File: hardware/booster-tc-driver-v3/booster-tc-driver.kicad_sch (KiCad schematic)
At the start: 98 parts, among them IC1 CAT4109V-GT2, IC2 LDL1117S50R, J1 62201021121, J11 3-647166-5, J2 EHT-105-01-S-D, J3 22-23-2021, J4 3-647166-2, J5 3-647166-2, J6 3-647166-2, J7 3-647166-2, Q1 T2N7002AK, Q2 BUK9M5R2-30EX, SW1 SW_SPDT, U1 IF-D95T << must be T, U2 IF-E96E, U3 IF-D95T << must be T, U4 CSTNE8M00G550000R0, U5 STM32G474CBTx, U6 MCP9700Ax-ETT, U7 AP1501A-12K5G-13, U8 LT1963AxST-3.3

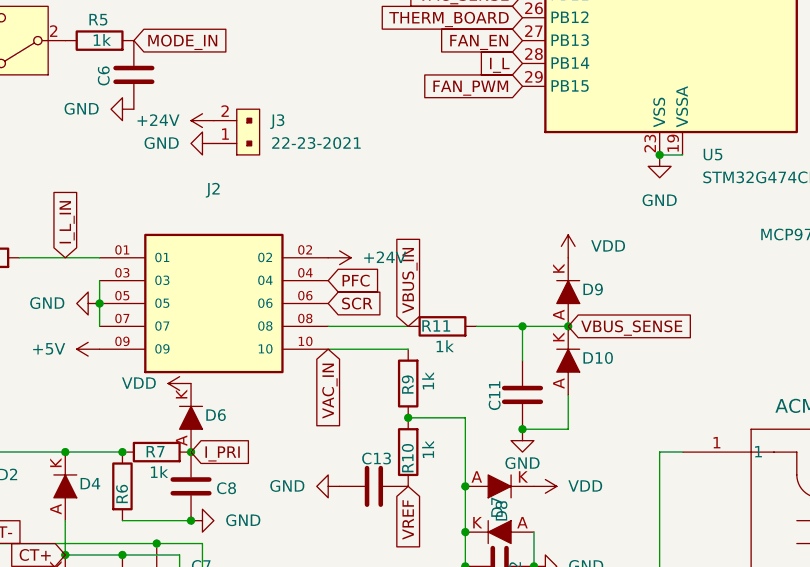
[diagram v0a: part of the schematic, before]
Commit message: pfc v3
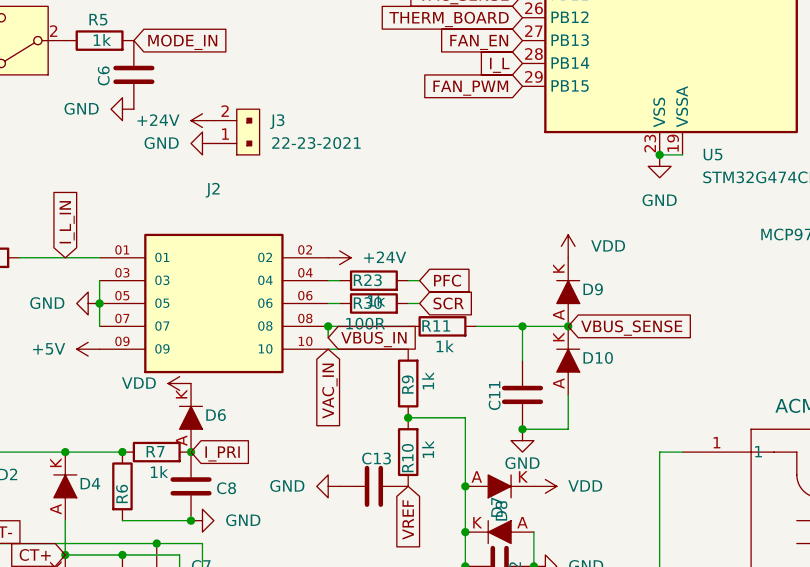
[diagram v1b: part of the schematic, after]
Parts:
- added R23: 1k, Resistor_SMD:R_0603_1608Metric_Pad0.98x0.95mm_HandSolder, symbol Device:R
- added R30: 100R, Resistor_SMD:R_0603_1608Metric_Pad0.98x0.95mm_HandSolder, symbol Device:R
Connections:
- net PFC: now also R23.2; no longer J2.04
- net SCR: now also R30.2; no longer J2.06
- new net: J2.06, R30.1
- new net: J2.04, R23.1
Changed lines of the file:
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@@
 	)
 	(junction
+		(at 62.23 160.02)
+		(diameter 0)
+		(color 0 0 0 0)
+	)
+	(junction
 		(at 36.83 53.34)
 		(diameter 0)
@@
 	(wire
 		(pts
+			(xy 71.12 157.48) (xy 72.39 157.48)
+		)
+		(stroke
+			(width 0)
+			(type default)
+		)
+	)
+	(wire
+		(pts
 			(xy 50.8 39.37) (xy 50.8 44.45)
 		)
@@
 	(wire
 		(pts
+			(xy 71.12 154.94) (xy 72.39 154.94)
+		)
+		(stroke
+			(width 0)
+			(type default)
+		)
+	)
+	(wire
+		(pts
 			(xy 99.06 140.97) (xy 101.6 140.97)
 		)
@@
 	(wire
 		(pts
+			(xy 62.23 157.48) (xy 63.5 157.48)
+		)
+		(stroke
+			(width 0)
+			(type default)
+		)
+	)
+	(wire
+		(pts
 			(xy 142.24 83.82) (xy 147.32 83.82)
 		)
@@
 	(wire
 		(pts
+			(xy 62.23 160.02) (xy 62.23 161.29)
+		)
+		(stroke
+			(width 0)
+			(type default)
+		)
+	)
+	(wire
+		(pts
 			(xy 39.37 181.61) (xy 46.99 181.61)
 		)
@@
 	(wire
 		(pts
+			(xy 62.23 154.94) (xy 63.5 154.94)
+		)
+		(stroke
+			(width 0)
+			(type default)
+		)
+	)
+	(wire
+		(pts
 			(xy 45.72 194.31) (xy 45.72 185.42)
 		)
@@
 		)
 	)
+	(global_label "PFC"
+		(shape input)
+		(at 72.39 154.94 0)
+		(fields_autoplaced yes)
+		(effects
+			(font
+				(size 1.27 1.27)
+			)
+			(justify left)
+		)
+		(property "Intersheetrefs" "${INTERSHEET_REFS}"
+			(at 79.0038 154.94 0)
+			(effects
+				(font
+					(size 1.27 1.27)
+				)
+				(justify left)
+				(hide yes)
+			)
+		)
+	)
 	(global_label "USART_TX"
 		(shape input)
@@
 		)
 	)
-	(global_label "VBUS_IN"
+	(global_label "SCR"
 		(shape input)
-		(at 71.12 160.02 90)
+		(at 72.39 157.48 0)
 		(fields_autoplaced yes)
 		(effects
@@
 		)
 		(property "Intersheetrefs" "${INTERSHEET_REFS}"
-			(at 71.12 149.2333 90)
+			(at 79.1247 157.48 0)
 			(effects
 				(font
@@
 		)
 	)
-	(global_label "SCR"
-		(shape input)
-		(at 62.23 157.48 0)
-		(fields_autoplaced yes)
-		(effects
-			(font
-				(size 1.27 1.27)
-			)
-			(justify left)
-		)
-		(property "Intersheetrefs" "${INTERSHEET_REFS}"
-			(at 68.9647 157.48 0)
-			(effects
-				(font
-					(size 1.27 1.27)
-				)
-				(justify left)
-				(hide yes)
-			)
-		)
-	)
-	(global_label "PFC"
-		(shape input)
-		(at 62.23 154.94 0)
-		(fields_autoplaced yes)
-		(effects
-			(font
-				(size 1.27 1.27)
-			)
-			(justify left)
-		)
-		(property "Intersheetrefs" "${INTERSHEET_REFS}"
-			(at 68.8438 154.94 0)
-			(effects
-				(font
-					(size 1.27 1.27)
-				)
-				(justify left)
-				(hide yes)
-			)
-		)
-	)
 	(global_label "VBUS_SENSE"
 		(shape input)
@@
 		)
 	)
+	(global_label "VBUS_IN"
+		(shape input)
+		(at 62.23 161.29 0)
+		(fields_autoplaced yes)
+		(effects
+			(font
+				(size 1.27 1.27)
+			)
+			(justify left)
+		)
+		(property "Intersheetrefs" "${INTERSHEET_REFS}"
+			(at 73.0167 161.29 0)
+			(effects
+				(font
+					(size 1.27 1.27)
+				)
+				(justify left)
+				(hide yes)
+			)
+		)
+	)
 	(symbol
 		(lib_id "Device:C")
@@
 	)
 	(symbol
+		(lib_id "Device:R")
+		(at 67.31 157.48 90)
+		(unit 1)
+		(exclude_from_sim no)
+		(in_bom yes)
+		(on_board yes)
+		(dnp no)
+		(property "Reference" "R30"
+			(at 68.326 157.48 90)
+			(effects
+				(font
+					(size 1.27 1.27)
+				)
+				(justify left)
+			)
+		)
+		(property "Value" "100R"
+			(at 68.58 159.766 90)
+			(effects
+				(font
+					(size 1.27 1.27)
+				)
+				(justify left)
+			)
+		)
+		(property "Footprint" "Resistor_SMD:R_0603_1608Metric_Pad0.98x0.95mm_HandSolder"
+			(at 67.31 159.258 90)
+			(effects
+				(font
+					(size 1.27 1.27)
+				)
+				(hide yes)
+			)
+		)
+		(property "Datasheet" "~"
+			(at 67.31 157.48 0)
+			(effects
+				(font
+					(size 1.27 1.27)
+				)
+				(hide yes)
+			)
+		)
+		(property "Description" "Resistor"
+			(at 67.31 157.48 0)
+			(effects
+				(font
+					(size 1.27 1.27)
+				)
+				(hide yes)
+			)
+		)
+		(pin "1"
+		)
+		(pin "2"
+		)
+		(instances
+			(project "booster-tc-driver"
+				(path "/3c175d5e-f31a-4933-a865-8318878a5034"
+					(reference "R30")
+					(unit 1)
+				)
+			)
+		)
+	)
+	(symbol
 		(lib_id "Device:C")
 		(at 46.99 177.8 0)
@@
 					(unit 1)
 				)
+			)
+		)
+	)
+	(symbol
+		(lib_id "Device:R")
+		(at 67.31 154.94 90)
+		(unit 1)
+		(exclude_from_sim no)
+		(in_bom yes)
+		(on_board yes)
+		(dnp no)
+		(property "Reference" "R23"
+			(at 68.326 154.94 90)
+			(effects
+				(font
+					(size 1.27 1.27)
+				)
+				(justify left)
+			)
+		)
+		(property "Value" "1k"
+			(at 68.58 157.226 90)
+			(effects
+				(font
+					(size 1.27 1.27)
+				)
+				(justify left)
+			)
+		)
+		(property "Footprint" "Resistor_SMD:R_0603_1608Metric_Pad0.98x0.95mm_HandSolder"
+			(at 67.31 156.718 90)
+			(effects
+				(font
+					(size 1.27 1.27)
+				)
+				(hide yes)
+			)
+		)
+		(property "Datasheet" "~"
+			(at 67.31 154.94 0)
+			(effects
+				(font
+					(size 1.27 1.27)
+				)
+				(hide yes)
+			)
+		)
+		(property "Description" "Resistor"
+			(at 67.31 154.94 0)
+			(effects
+				(font
+					(size 1.27 1.27)
+				)
+				(hide yes)
+			)
+		)
+		(pin "1"
+		)
+		(pin "2"
+		)
+		(instances
+			(project "booster-tc-driver"
+				(path "/3c175d5e-f31a-4933-a865-8318878a5034"
+					(reference "R23")
+					(unit 1)
+				)

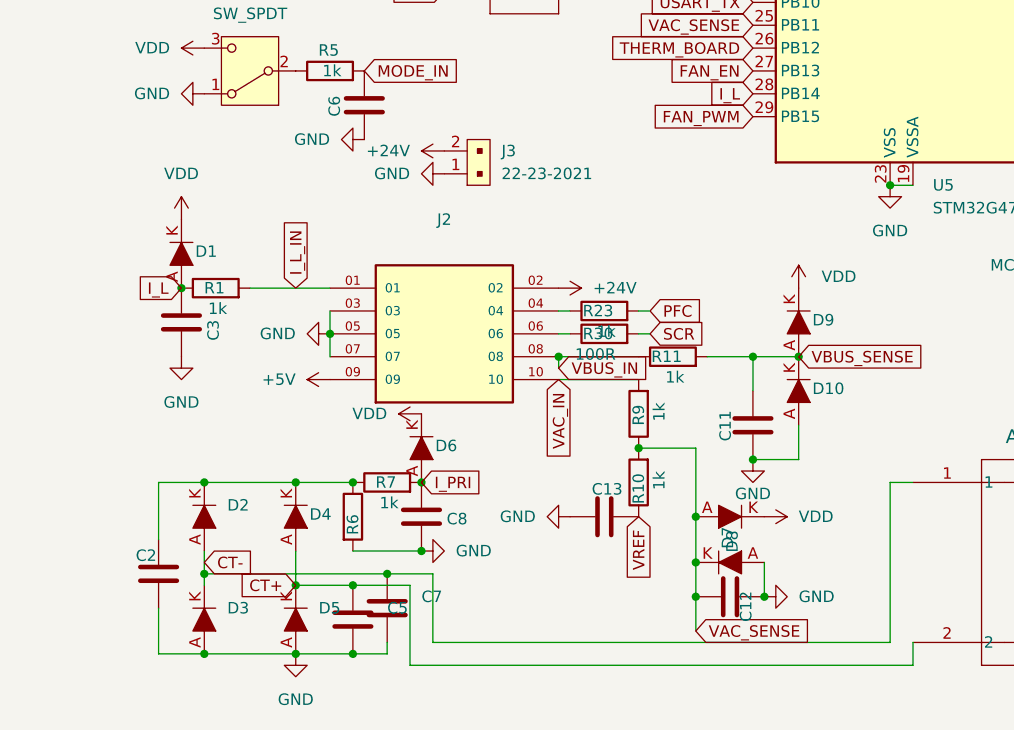
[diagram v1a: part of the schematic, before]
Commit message: pfc v3 finalized
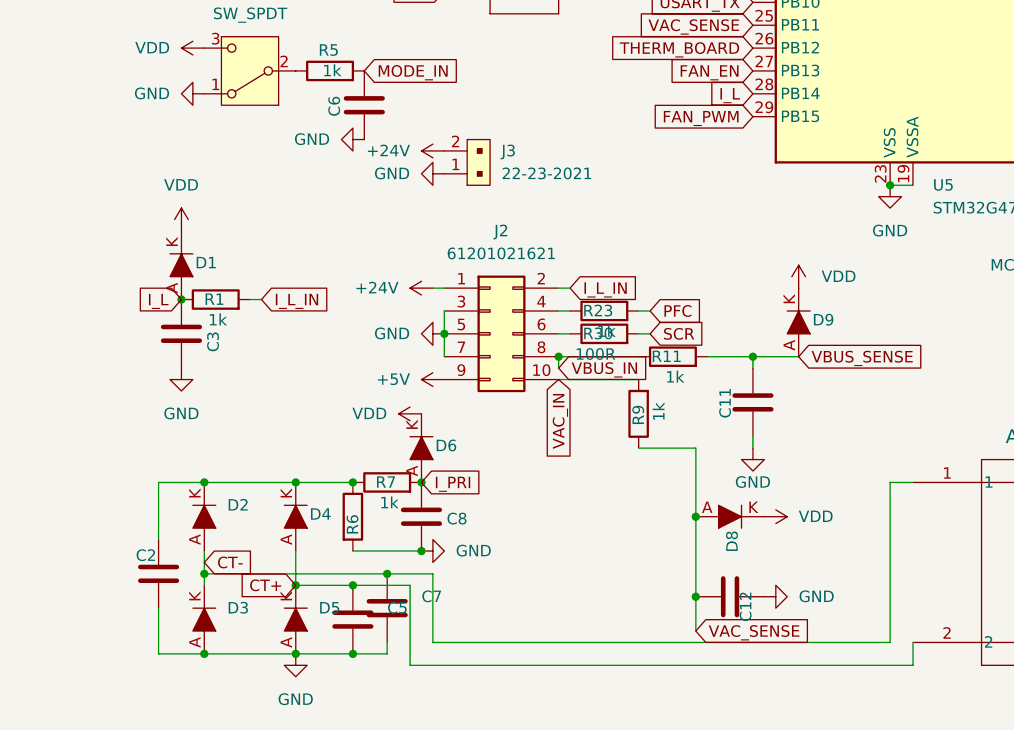
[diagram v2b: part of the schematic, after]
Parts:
- removed C13: .1uf, Capacitor_SMD:C_0603_1608Metric_Pad1.08x0.95mm_HandSolder, symbol Device:C
- removed D10, D7: 1N5819HW-7-F, digikey-footprints:SOD-123, symbol dk_Diodes-Rectifiers-Single:1N5819HW-7-F
- removed J2: EHT-105-01-S-D, Library:SAMTEC_EHT-105-01-S-D, symbol EHT-105-01-S-D:EHT-105-01-S-D
- removed R10: 1k, Resistor_SMD:R_0603_1608Metric_Pad0.98x0.95mm_HandSolder, symbol Device:R
- added J2: 61201021621, Connector_IDC:IDC-Header_2x05_P2.54mm_Vertical, symbol Connector_Generic:Conn_02x05_Odd_Even
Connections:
- net +24V: now also J2.1 (Pin_1)
- net +5V: now also J2.9 (Pin_9)
- net GND: now also J2.3 (Pin_3), J2.5 (Pin_5), J2.7 (Pin_7)
- net I_L_IN: now also J2.2 (Pin_2)
- net VAC_IN: now also J2.10 (Pin_10)
- net VBUS_IN: now also J2.8 (Pin_8)
- net at R30.1: now also J2.6 (Pin_6)
- net at R23.1: now also J2.4 (Pin_4)
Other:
- moved on the sheet: C11, C3, D1, R1

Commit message: idk
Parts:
- C6, C9: value 1u -> 2u2
